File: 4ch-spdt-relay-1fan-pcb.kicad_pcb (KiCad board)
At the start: 2 copper layers, 107.9 x 62.8 mm, 49 parts, among them J1 Screw_Terminal_01x03, J2 Conn_01x08_Pin, J3 Screw_Terminal_01x03, J4 Screw_Terminal_01x03, J5 Screw_Terminal_01x03, K1 G5LE-1, K2 G5LE-1, K3 G5LE-1, K4 G5LE-1, Q1 2N3904, Q2 2N3904, Q3 2N3904, Q4 2N3904, Q5 BT136, U5 MOC3021M, U6 PC817

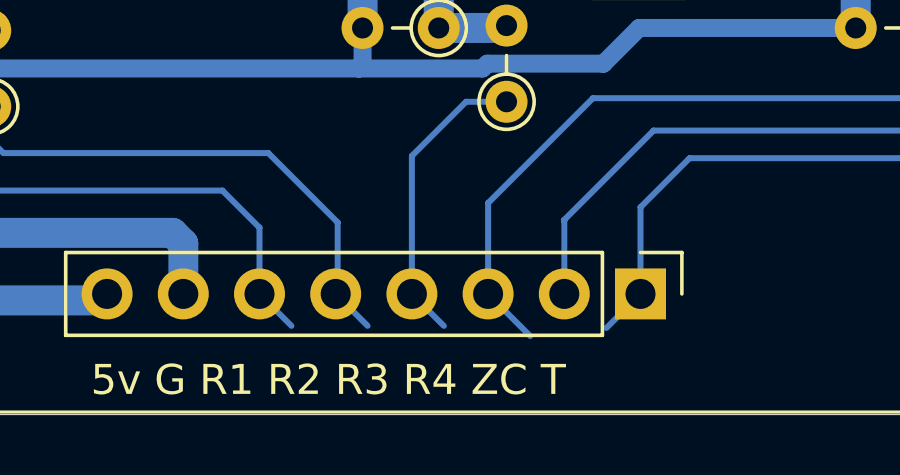
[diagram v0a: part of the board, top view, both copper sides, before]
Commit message: Add files via upload
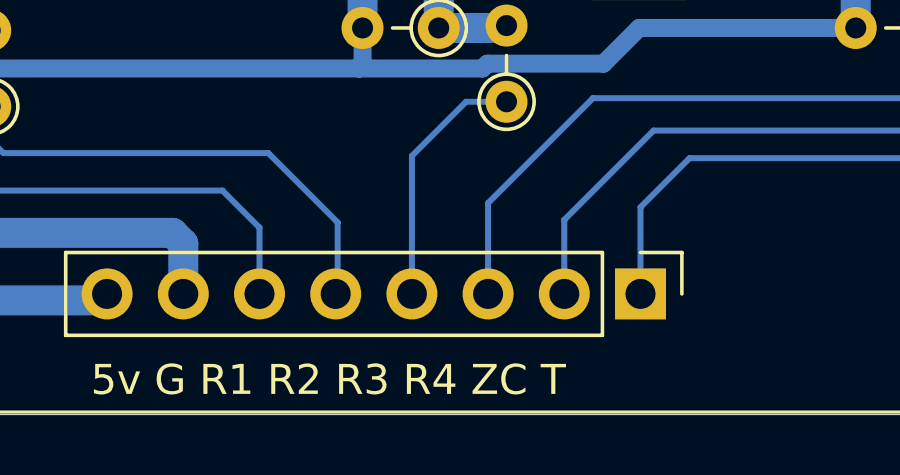
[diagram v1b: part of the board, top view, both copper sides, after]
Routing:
- net Net-(J2-Pin_3): track 23.5 -> 21.5 mm
- net Net-(J2-Pin_1): track 28.5 -> 26.9 mm
- net Net-(J2-Pin_6): track 32.1 -> 30.6 mm
- net Net-(J2-Pin_5): track 17.7 -> 16.2 mm
- net Net-(J2-Pin_4): track 10.0 -> 8.50 mm
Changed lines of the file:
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@@
 		(filling no)
 		(pcbplotparams
-			(layerselection 0x00000000_00000000_55555555_5555557d)
+			(layerselection 0x00000000_00000000_5555555d_5755557d)
 			(plot_on_all_layers_selection 0x00000000_00000000_00000000_00000000)
 			(disableapertmacros no)
@@
 			(crossoutdnponfab yes)
 			(subtractmaskfromsilk no)
-			(outputformat 4)
+			(outputformat 1)
 			(mirror no)
-			(drillshape 2)
+			(drillshape 0)
 			(scaleselection 1)
 			(outputdirectory "")
@@
 	)
 	(segment
-		(start 114.355 86.425)
-		(end 115.42 87.49)
-		(width 0.2)
-		(layer "B.Cu")
-		(net "Net-(J2-Pin_6)")
-	)
-	(segment
 		(start 104.95 82.98)
 		(end 113.12 82.98)
@@
 	)
 	(segment
-		(start 121.975 86.425)
-		(end 123.38 87.83)
-		(width 0.2)
-		(layer "B.Cu")
-		(net "Net-(J2-Pin_3)")
-	)
-	(segment
 		(start 125.47 79.9)
 		(end 121.975 83.395)
@@
 	)
 	(segment
-		(start 127.055 86.425)
-		(end 125.92 87.56)
-		(width 0.2)
-		(layer "B.Cu")
-		(net "Net-(J2-Pin_1)")
-	)
-	(segment
 		(start 138.905 37.9675)
 		(end 138.905 64.115)
@@
 	)
 	(segment
-		(start 119.435 86.425)
-		(end 120.5 87.49)
-		(width 0.2)
-		(layer "B.Cu")
-		(net "Net-(J2-Pin_4)")
-	)
-	(segment
 		(start 121.24 80.02)
 		(end 119.435 81.825)
@@
 		(width 0.2)
 		(layer "B.Cu")
-		(net "Net-(J2-Pin_5)")
-	)
-	(segment
-		(start 116.895 86.425)
-		(end 117.96 87.49)
-		(width 0.2)
-		(layer "B.Cu")
